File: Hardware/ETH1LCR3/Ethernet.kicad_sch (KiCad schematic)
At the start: 33 parts, among them J201 RJ45_Abracon_ARJP11A-MASA-B-A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, U201 LAN8742A, U202 Ag9905LP, Y201 NX5032GA-25

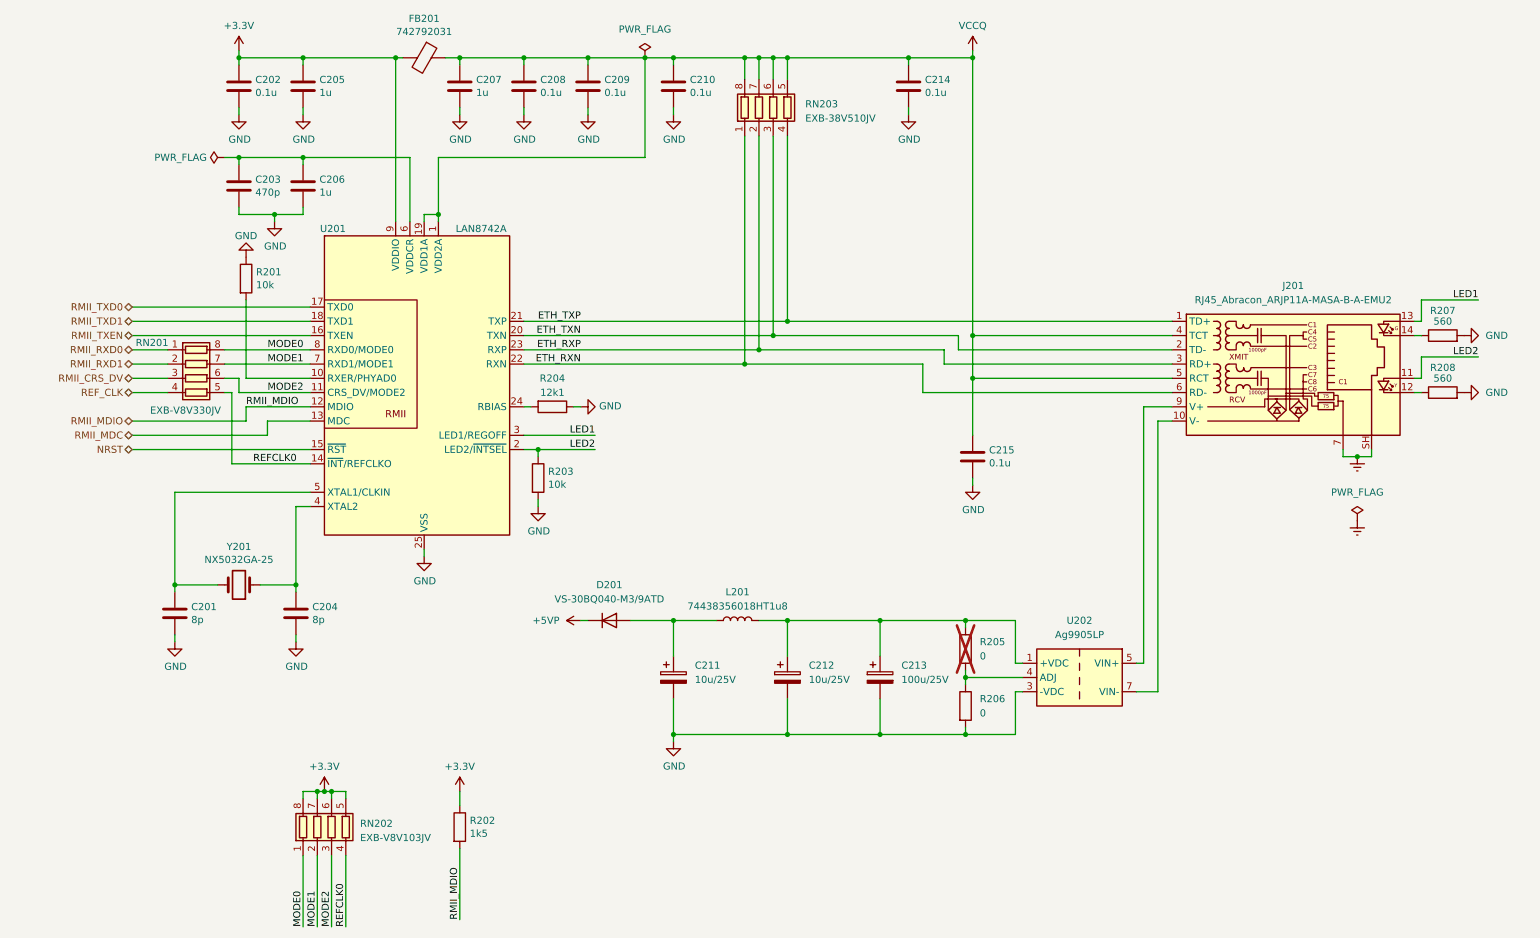
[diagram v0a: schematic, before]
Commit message: Hardware
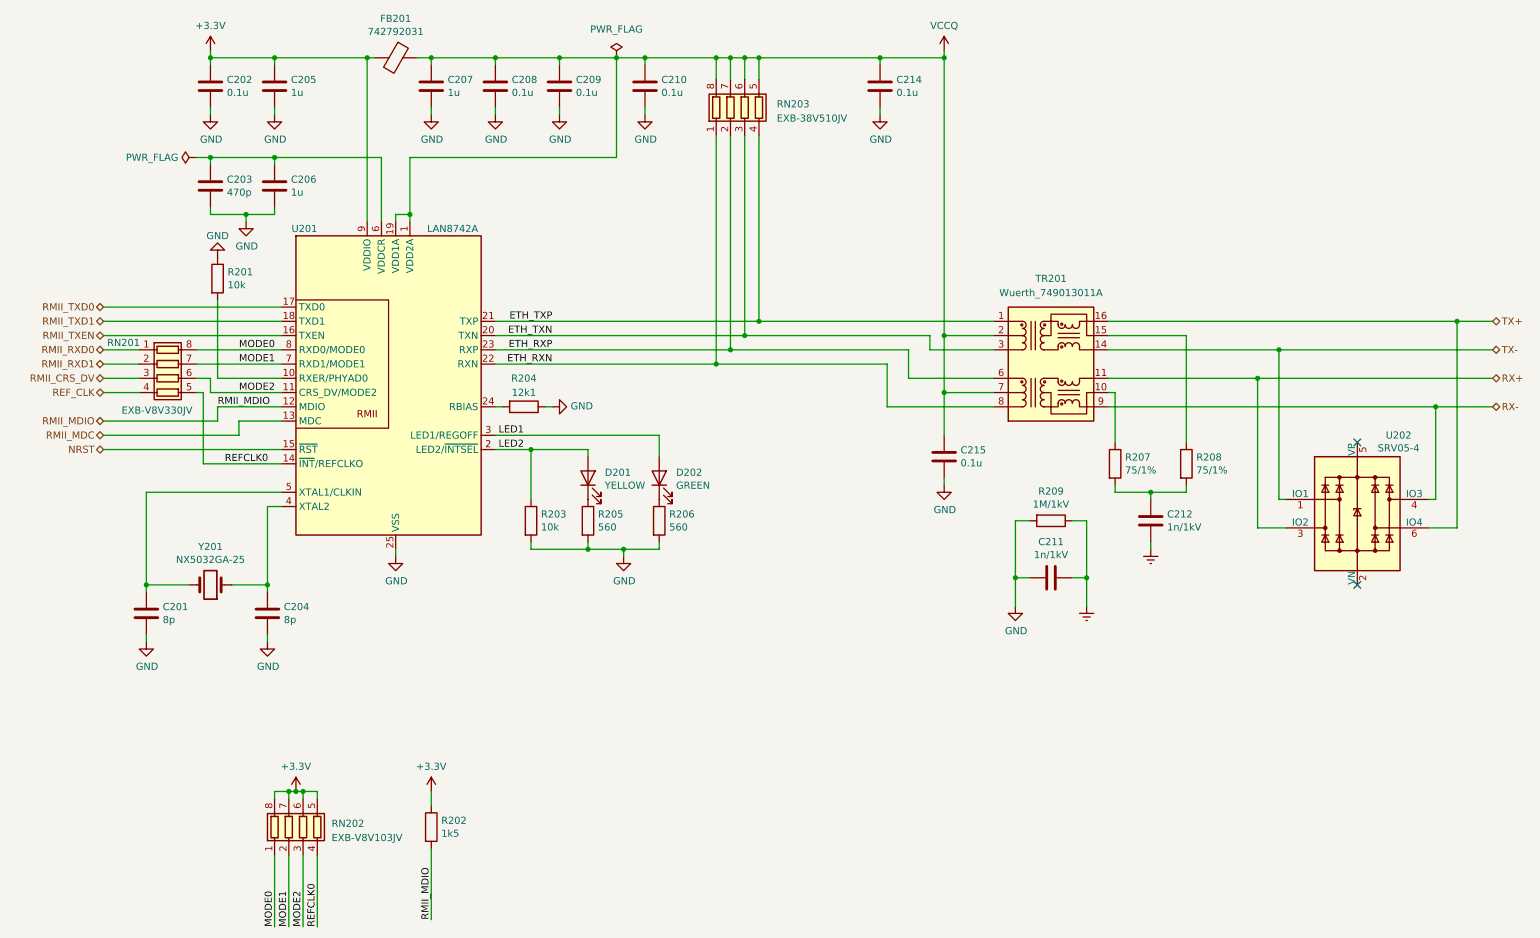
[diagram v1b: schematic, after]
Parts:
- removed C211, C212: 10u/25V, symbol Device:C_Polarized
- removed C213: 100u/25V, symbol Device:C_Polarized
- removed D201: VS-30BQ040-M3/9ATD, symbol Device:D
- removed J201: RJ45_Abracon_ARJP11A-MASA-B-A-EMU2, Connector_RJ:RJ45_Abracon_ARJP11A-MA_Horizontal, symbol Connector:RJ45_Abracon_ARJP11A-MASA-B-A-EMU2
- removed L201: 74438356018HT1u8, symbol Device:L
- removed U202: Ag9905LP, Converter_DCDC:Converter_DCDC_Silvertel_Ag99xxLP_THT, symbol Converter_DCDC:Ag9905LP
- added C211, C212: 1n/1kV, symbol Device:C
- added D201: YELLOW, LED_SMD:LED_0603_1608Metric_Pad1.05x0.95mm_HandSolder, symbol Device:LED
- added D202: GREEN, LED_SMD:LED_0603_1608Metric_Pad1.05x0.95mm_HandSolder, symbol Device:LED
- added R209: 1M/1kV, Resistor_SMD:R_1206_3216Metric_Pad1.30x1.75mm_HandSolder, symbol Device:R
- added TR201: Wuerth_749013011A, Transformer_SMD:Transformer_Ethernet_Wuerth_749013011A, symbol Transformer:Wuerth_749013011A
- added U202: SRV05-4, Converter_DCDC:Converter_DCDC_Silvertel_Ag99xxLP_THT, symbol Power_Protection:SRV05-4
- R205: value 0 -> 560; now fitted; now in the parts list
- R206: value 0 -> 560
- R207, R208: value 560 -> 75/1%
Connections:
- net ETH_RXN: now also TR201.8 (RD-)
- net ETH_RXP: now also TR201.6 (RD+)
- net ETH_TXN: now also TR201.3 (TD-)
- net ETH_TXP: now also TR201.1 (TD+)
- net Earth: now also C211.1, C212.2, R209.1
- net GND: now also R205.2, C211.2, R209.2; no longer R207.2, R208.2
- net LED1: now also D202.2 (A)
- net LED2: now also D201.2 (A)
- net VCCQ: now also TR201.2 (C_TD), TR201.7 (C_RD)
- net at R205.1: now also D201.1 (K)
- net at R207.1: now also TR201.10 (C_RX)
- net at R208.1: now also TR201.15 (C_TX)
- net at R206.1: now also D202.1 (K); no longer R205.2
- new net: C212.1, R207.2, R208.2
- new net RX+: TR201.11 (RX+), U202.3 (IO2)
- new net RX-: TR201.9 (RX-), U202.4 (IO3)
- new net TX+: TR201.16 (TX+), U202.6 (IO4)
- new net TX-: TR201.14 (TX-), U202.1 (IO1)
- no-connect marks 0 -> 2
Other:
- moved on the sheet: C201, C202, C203, C204, C205, C206, C207, C208, C209, C210, C214, C215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
